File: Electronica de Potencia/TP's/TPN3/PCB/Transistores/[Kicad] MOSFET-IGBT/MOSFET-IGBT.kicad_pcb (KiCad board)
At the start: 2 copper layers, 70.9 x 52.3 mm, 20 parts, among them J1 Vin, J2 PWM_IN, Q1 FGPF7N60RUFD, Q2 IRF840, T1 50:50

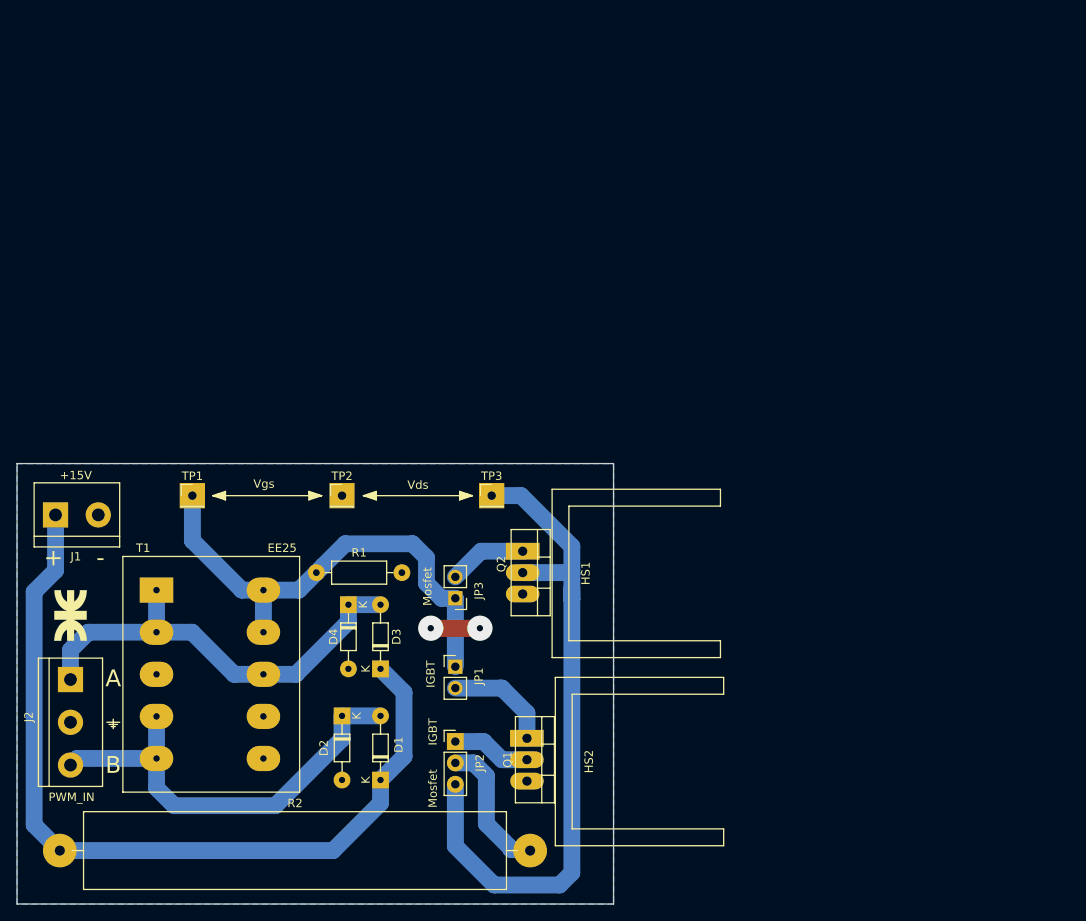
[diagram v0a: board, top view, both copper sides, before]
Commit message: Arreglo placa de potencia
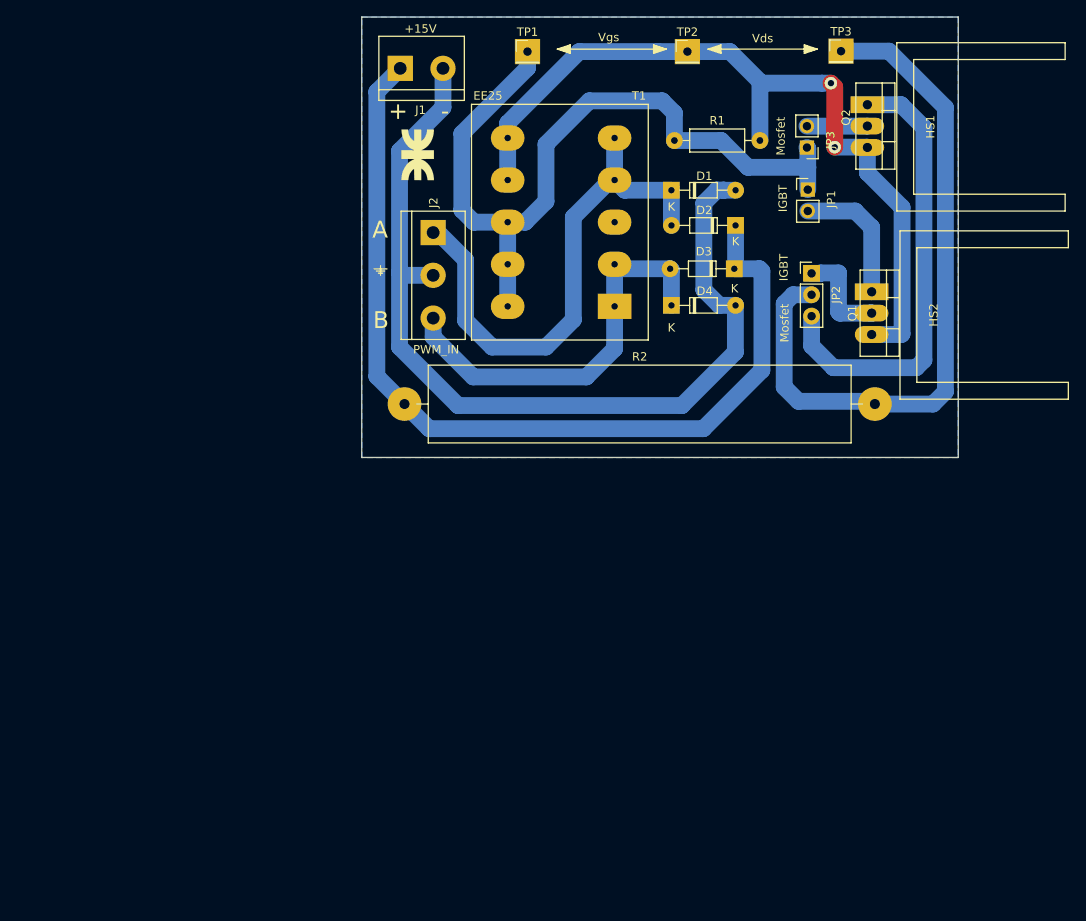
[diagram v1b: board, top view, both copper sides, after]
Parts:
- JP1: value IGBT -> Jumper_NC_Small
- JP2: value MOSFET O IGBT -> Jumper_NC_Dual
- JP3: value MOSFET -> Jumper_NC_Small
- TP3: value TP_VDS -> TP_VCE_VDS
- moved D1 78.2 mm to (159.0, 92.1), turned to 180 degrees
- moved D2 73.7 mm to (151.4, 87.9), turned to 0 degrees
- moved JP1 70.5 mm to (167.6, 87.8)
- moved JP2 69.9 mm to (168.1, 97.8)
- moved G1 68.5 mm to (121.2, 83.7)
- moved J2 68.4 mm to (123.1, 92.9)
- moved JP3 67.9 mm to (167.5, 82.8)
- moved TP3 67.2 mm to (171.6, 71.4)
- moved J1 67.0 mm to (119.2, 73.4)
- moved Q2 67.0 mm to (174.7, 77.8)
- moved R2 67.0 mm to (119.7, 113.3)
- moved HS1 67.0 mm to (198.2, 70.4)
- moved HS2 67.0 mm to (198.6, 92.7)
- moved Q1 67.0 mm to (175.2, 100.0)
- moved TP2 66.8 mm to (153.3, 71.5)
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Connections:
- J2 pad 1: /PWM_A -> /PWM_B
- J2 pad 3: /PWM_B -> /PWM_A
- Q1 pad 3: GND -> Earth
- Q2 pad 1: Net-(JP3-Pad2) -> Net-(JP2-Pad3)
- Q2 pad 2: Net-(JP2-Pad3) -> Net-(JP3-Pad2)
- Q2 pad 3: GND -> Earth
- R1 pad 2: GND -> Earth
- T1 pad : /PWM_A -> Net-(JP1-Pad1)
- T1 pad 3: GND -> Earth
- TP2 pad 1: GND -> Earth
- TP3 pad 1: Net-(JP2-Pad3) -> Net-(JP2-Pad2)
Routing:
- net GND: track 5.84 -> 109.6 mm, vias 2 -> 0
- net Earth: track 0.00 -> 96.4 mm, vias 0 -> 2
- net Net-(JP2-Pad2): track 16.6 -> 83.1 mm
- net Net-(JP1-Pad1): track 58.9 -> 93.9 mm
- net Net-(JP2-Pad3): track 81.3 -> 53.8 mm
- net /PWM_B: track 52.6 -> 63.2 mm
- net +15V: track 100.5 -> 109.3 mm
- net /PWM_A: track 52.9 -> 48.6 mm
- net Net-(JP1-Pad2): track 12.7 -> 16.0 mm
- net Net-(JP2-Pad1): track 9.40 -> 12.0 mm
- net Net-(JP3-Pad2): track 9.26 -> 7.19 mm
